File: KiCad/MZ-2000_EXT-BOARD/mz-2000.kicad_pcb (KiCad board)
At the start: 2 copper layers, 100 x 99.8 mm, 5 parts, among them J1 Conn_02x22_Row_Letter_First, J2 Conn_02x22_Row_Letter_First, J4 Jack-DC, J5 Conn_02x22_Row_Letter_First

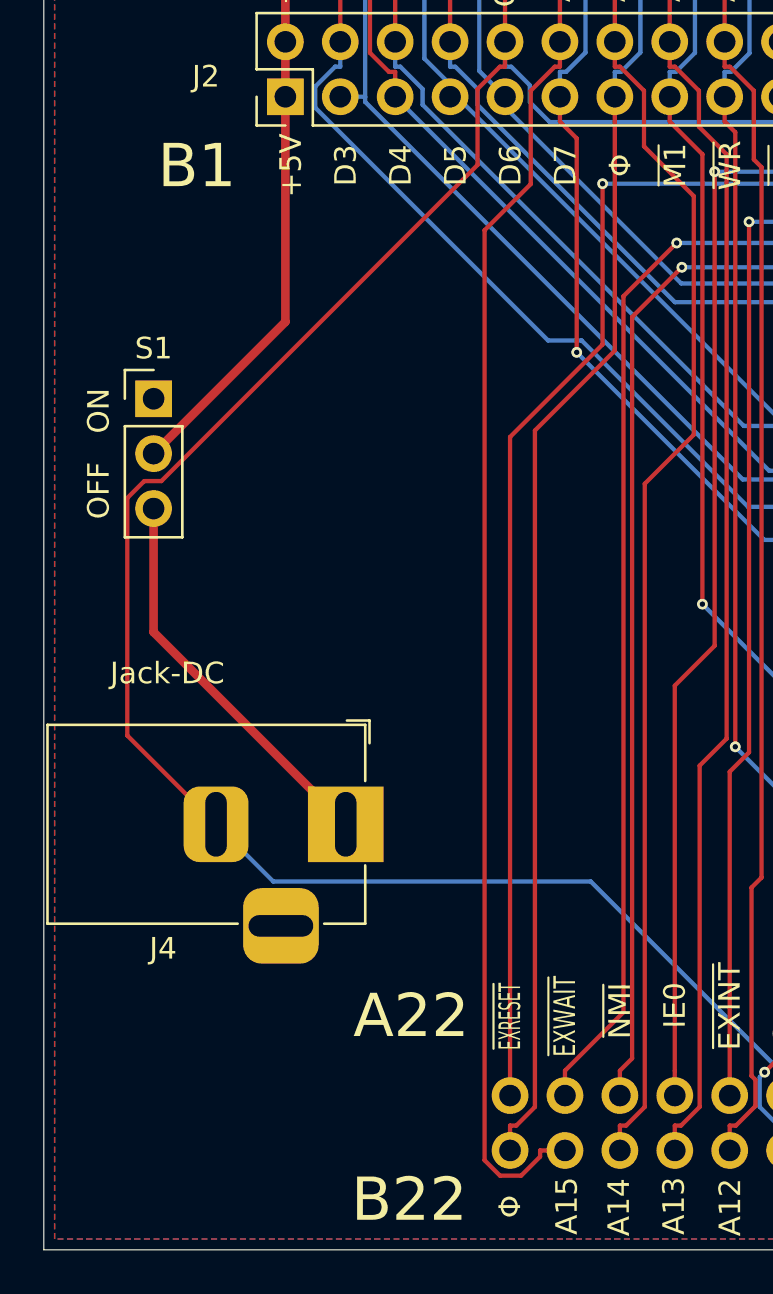
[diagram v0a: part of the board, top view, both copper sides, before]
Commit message: Add files via upload
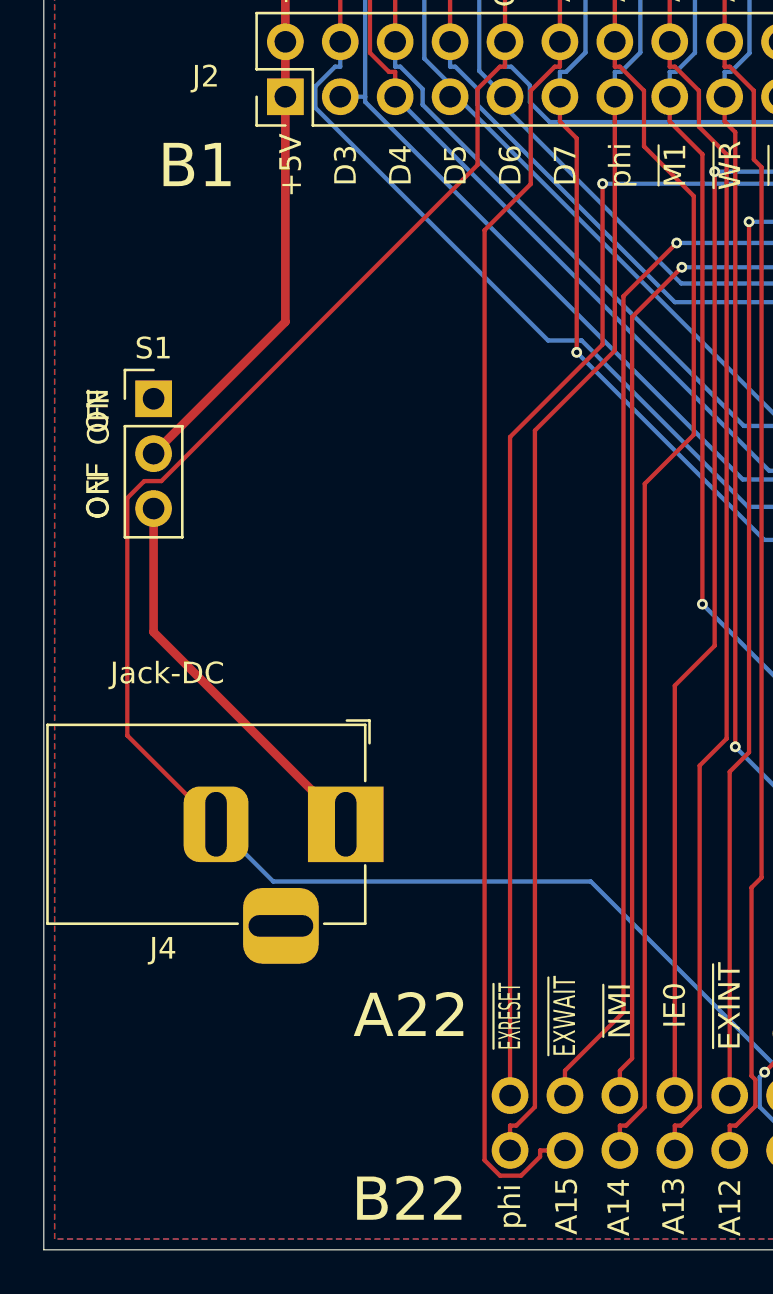
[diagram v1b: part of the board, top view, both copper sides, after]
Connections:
- net /Φ renamed /phi
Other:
- board text added: "ON OFF"
- board text added: "phi"
- board text removed: "Φ"
